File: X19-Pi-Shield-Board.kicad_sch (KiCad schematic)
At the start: 47 parts, among them IC1 STM32C542CCT6, J1 Raspberry_Pi_4, J2 Conn_01x02, J3 Conn_01x02, J4 Conn_01x04, J5 Conn_01x04, J6 Conn_01x03, J7 Conn_01x03, J8 Conn_02x05_Odd_Even, SW1 SW_Push, U1 MIC5504-3.3YM5, U2 BME280, U3 INA237AIDGSR, U4 TCAN1044VDRQ1, U5 MCP2518FDT-E/QBB, U6 TCAN1044VDRQ1, Y1 ECS-120-18-33-JGN-TR, Y2 ECS-120-18-33-JGN-TR

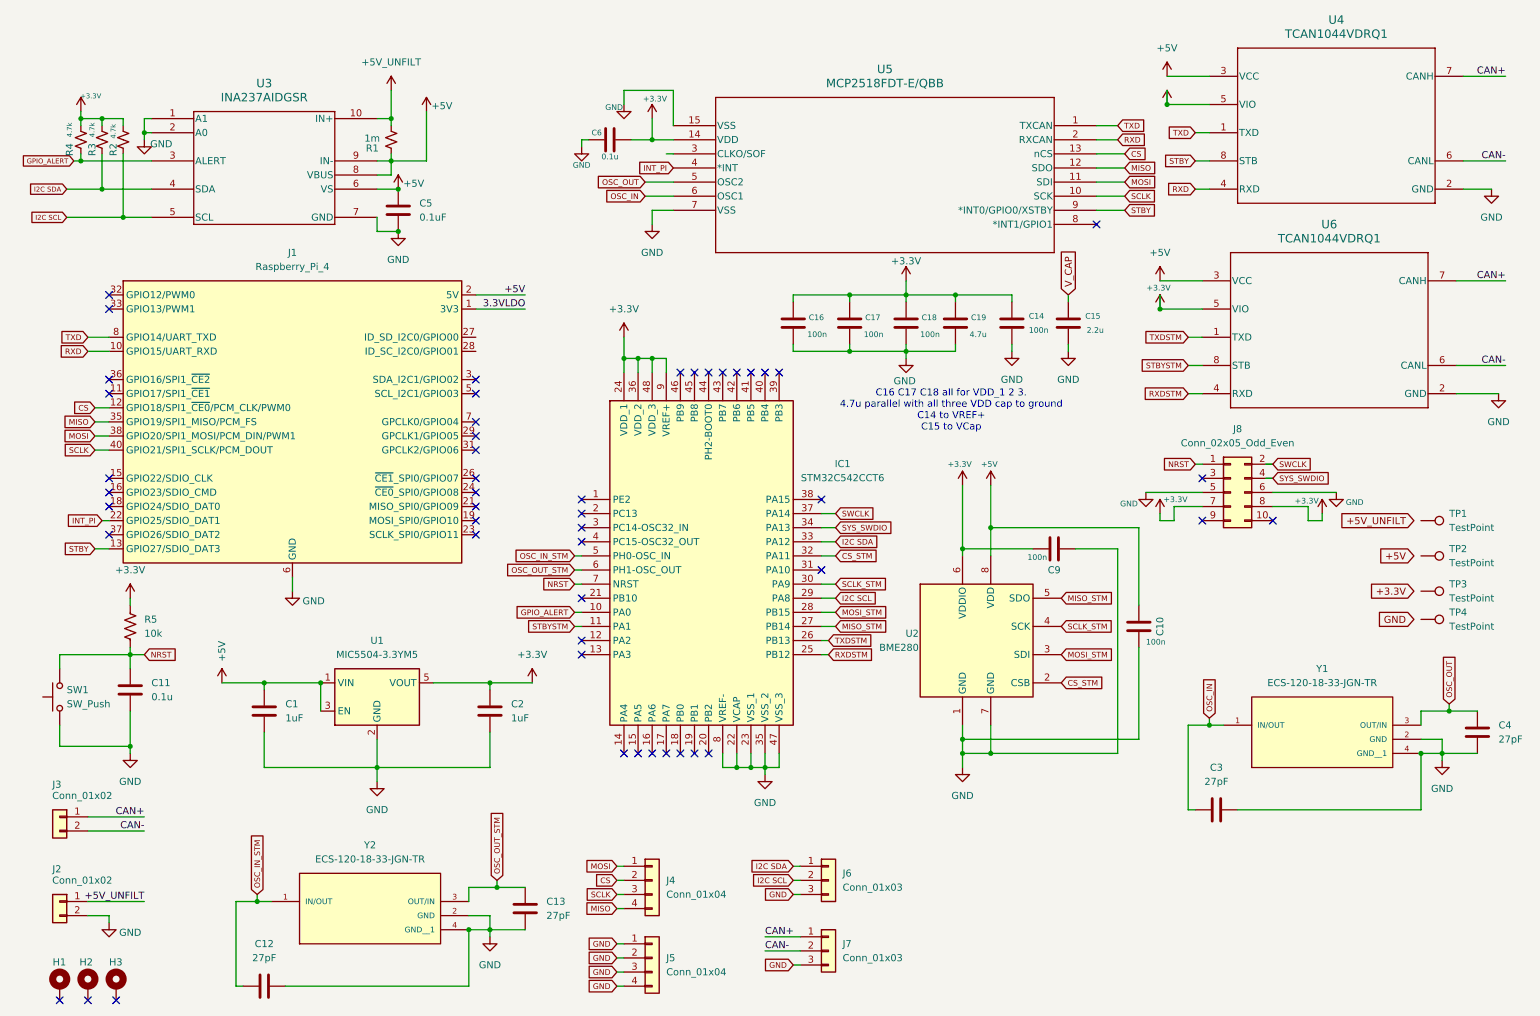
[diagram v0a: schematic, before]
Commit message: Pre Sch Review - Nick Changes
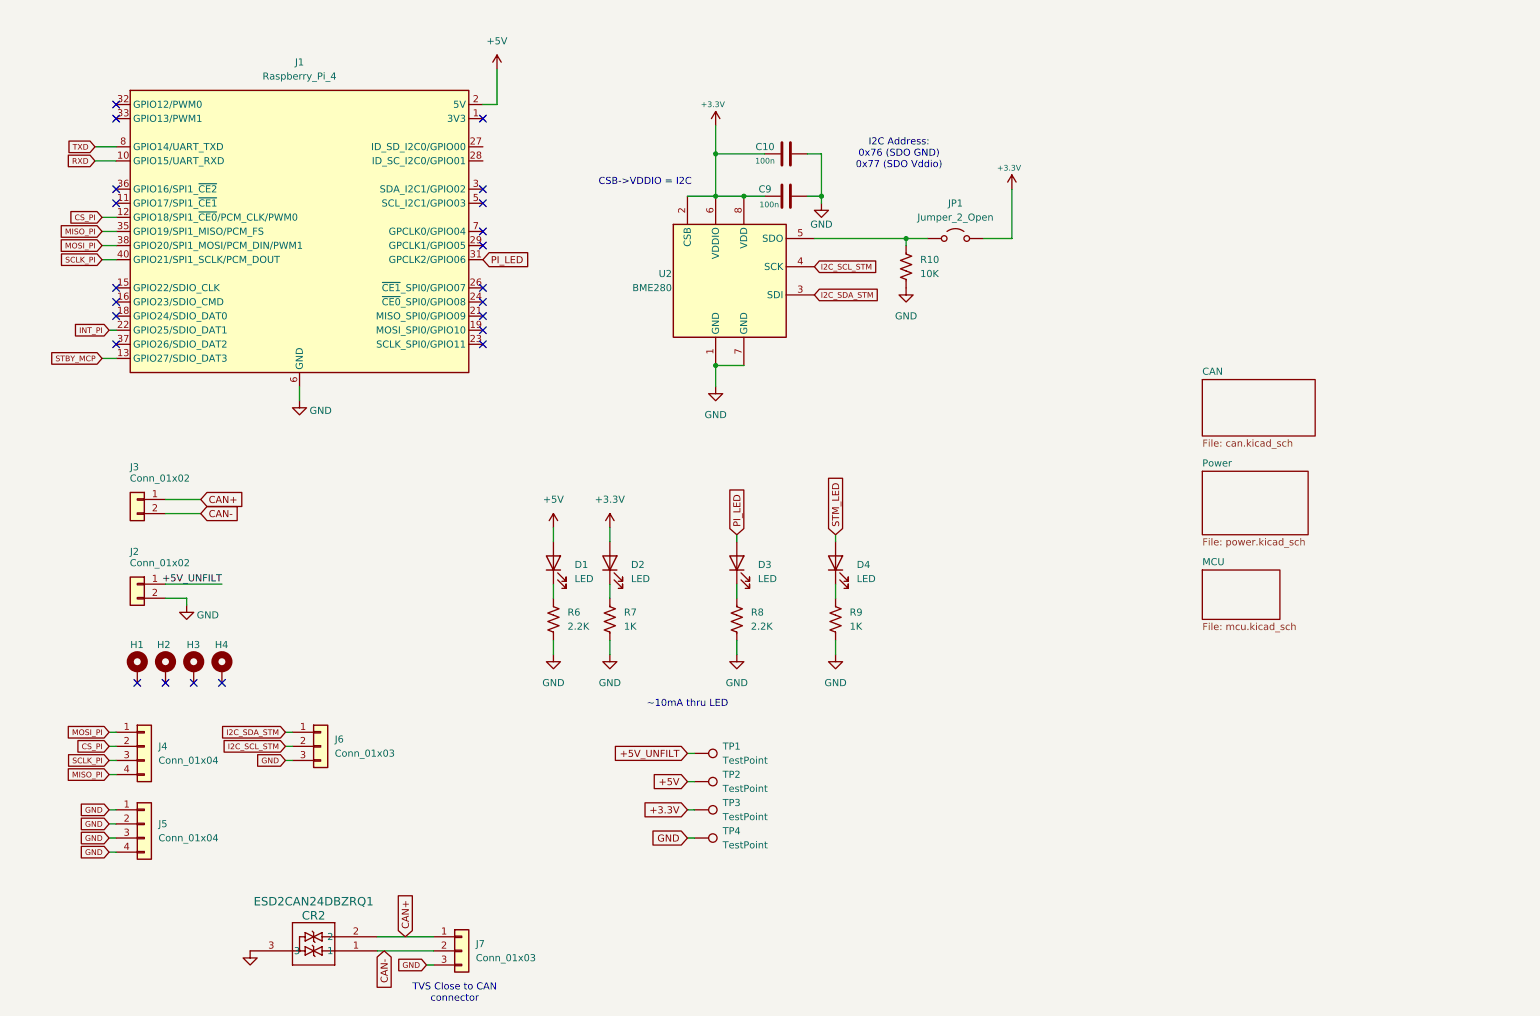
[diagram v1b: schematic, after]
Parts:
- removed C1, C2: 1uF, Package_SO:SOIC-8_3.9x4.9mm_P1.27mm, symbol Device:C
- removed C11, C6: 0.1u, symbol Device:C
- removed C12, C13, C3, C4: 27pF, symbol Device:C
- removed C14, C16, C17, C18: 100n, symbol Device:C
- removed C15: 2.2u, symbol Device:C
- removed C19: 4.7u, symbol Device:C
- removed C5: 0.1uF, symbol Device:C
- removed IC1: STM32C542CCT6, QFP50P900X900X160-48N, symbol STM32C542CCT6:STM32C542CCT6
- removed J8: Conn_02x05_Odd_Even, Oscillator:Oscillator_SMD_ECS_2520MV-xxx-xx-4Pin_2.5x2.0mm, symbol Connector_Generic:Conn_02x05_Odd_Even
- removed R1: 1m, D0008A-IPC_A, symbol Device:R_Small_US
- removed R2, R3, R4: 4.7k, symbol Device:R_Small_US
- removed R5: 10k, Resistor_THT:R_Array_SIP4, symbol Device:R_US
- removed SW1: SW_Push, Button_Switch_THT:SW_NKK_GW12LJP, symbol Switch:SW_Push
- removed U1: MIC5504-3.3YM5, Package_TO_SOT_SMD:SOT-23-5, symbol Regulator_Linear:MIC5504-3.3YM5
- removed U3: INA237AIDGSR, VSSOP_IDGSR_TEX, symbol INA237AIDGSR:INA237AIDGSR
- removed U4, U6: TCAN1044VDRQ1, D0008A-IPC_A, symbol TCAN1044VDRQ1:TCAN1044VDRQ1
- removed U5: MCP2518FDT-E/QBB, VDFN14_QBB_MCH, symbol MCP2518FDT_E_QBB:MCP2518FDT-E_QBB
- removed Y1, Y2: ECS-120-18-33-JGN-TR, ECS-120-18-33-JGN-TR:XTAL_ECS-120-18-33-JGN-TR, symbol ECS-120-18-33-JGN-TR:ECS-120-18-33-JGN-TR
- added CR2: ESD2CAN24DBZRQ1, SOT-23_DBZ_TEX, symbol board_control_manual_lib:ESD2CAN24DBZRQ1
- added D1, D2, D3, D4: LED, symbol Device:LED
- added H4: MountingHole_Pad, symbol Mechanical:MountingHole_Pad
- added JP1: Jumper_2_Open, symbol Jumper:Jumper_2_Open
- added R10: 10K, symbol Device:R_US
- added R6, R8: 2.2K, symbol Device:R_US
- added R7, R9: 1K, symbol Device:R_US
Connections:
- net CS_STM is gone; now on net +3.3V: U2.2 (CSB)
- net MOSI_STM is gone; now on net I2C_SDA_STM: U2.3 (SDI)
- net SCLK_STM is gone; now on net I2C_SCL_STM: U2.4 (SCK)
- net +3.3V: now also C10.2, TP3.1, U2.8 (VDD), D2.2 (A), JP1.2 (B)
- net +5V: now also TP2.1, D1.2 (A); no longer C10.2, U2.8 (VDD)
- net +5V_UNFILT: now also TP1.1
- net CAN+: now also CR2.2
- net CAN-: now also CR2.1
- net GND: now also TP4.1, CR2.3, R10.2, R6.2, R7.2, R8.2, R9.2
- net PI_LED: now reaches J1.31 (GPCLK2/GPIO06)
- net PI_LED: now also D3.2 (A)
- net 3.3VLDO: no longer names the net of J1.1 (3V3), J1.17 (3V3)
- net CS renamed CS_PI
- net I2C SCL renamed I2C_SCL_STM
- net I2C SDA renamed I2C_SDA_STM
- net MISO renamed MISO_PI
- net MISO_STM: no longer names the net of U2.5 (SDO)
- net MISO_STM: now also JP1.1 (A), R10.1
- net MOSI renamed MOSI_PI
- net SCLK renamed SCLK_PI
- net STBY renamed STBY_MCP
- new net: D2.1 (K), R7.1
- new net: D4.1 (K), R9.1
- new net: D1.1 (K), R6.1
- new net: D3.1 (K), R8.1
- new net STM_LED: D4.2 (A)
- no-connect marks 49 -> 22
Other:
- added sheet CAN (can.kicad_sch)
- added sheet MCU (mcu.kicad_sch)
- added sheet Power (power.kicad_sch)
- note added: "CSB->VDDIO = I2C"
- note added: "I2C Address: 0x76 (SDO GND) 0x77 (SDO Vddio)"
- note added: "TVS Close to CAN connector"
- note added: "~10mA thru LED"
- note removed: "C16 C17 C18 all for VDD_1 2 3. 4.7u parallel with all three VDD cap to ground C14 to VREF+ C15 to VCap"
- moved on the sheet: C10, C9, H1, H2, H3, J1, J2, J3, J4, J5, J6, J7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
